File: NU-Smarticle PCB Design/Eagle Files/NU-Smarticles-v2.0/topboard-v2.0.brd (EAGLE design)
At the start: 48 x 22 mm, 17 parts, among them CON1 LI-PO, CON2 12XFFCEXTEND, M1 SERVO, M2 SERVO, U1 XBEE3, U2 INA180B2

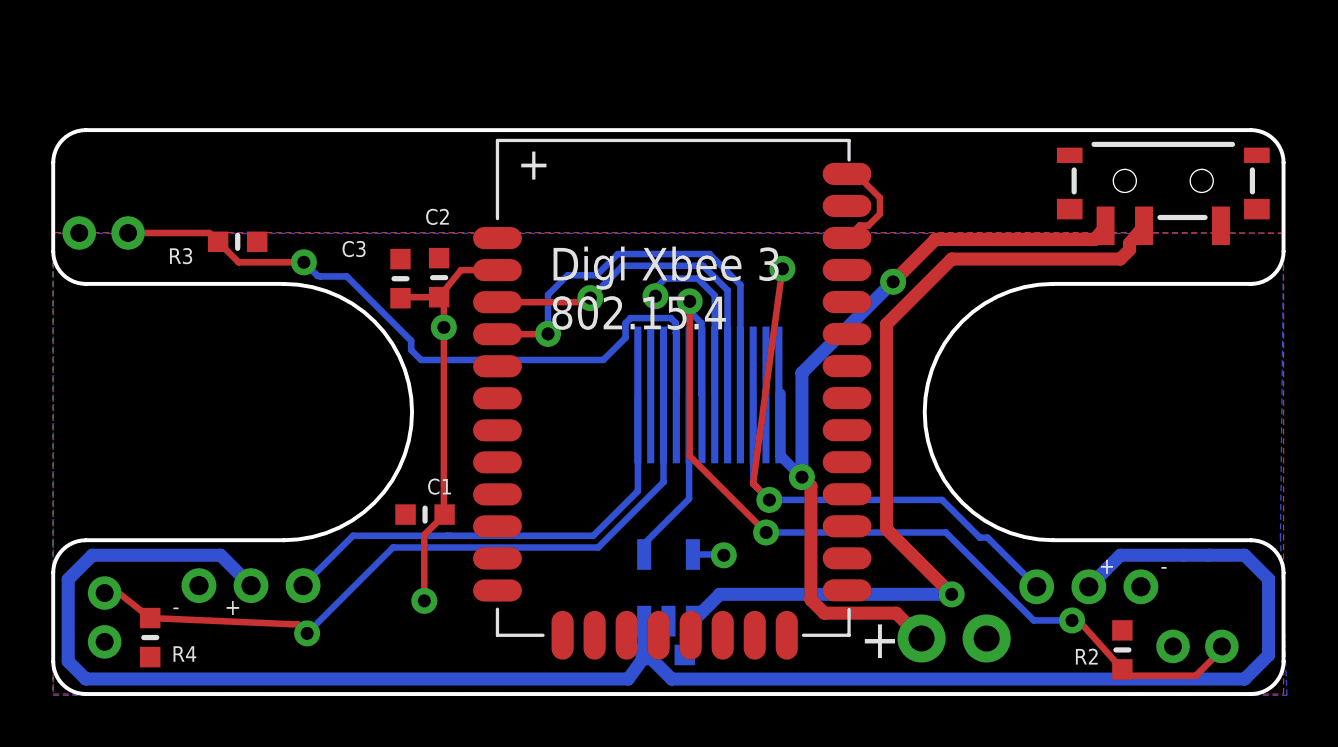
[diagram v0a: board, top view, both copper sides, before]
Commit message: eagle work and files added
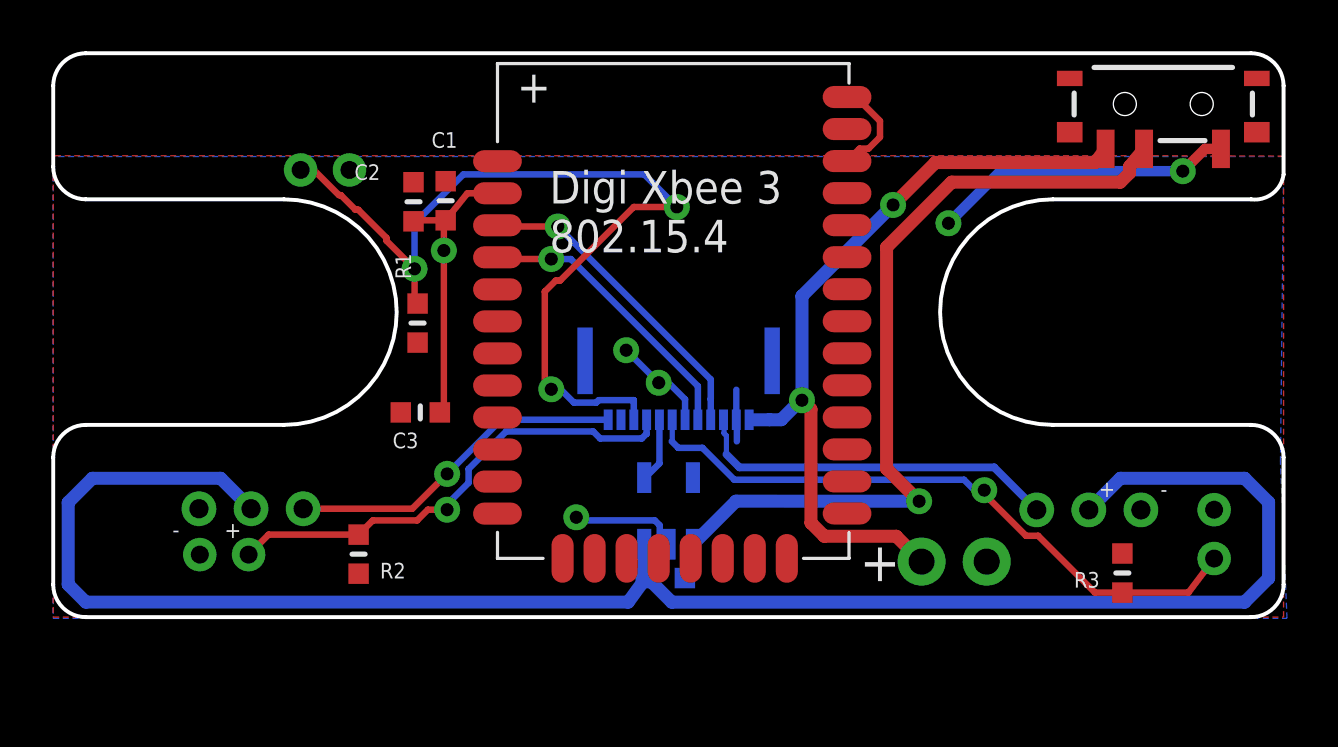
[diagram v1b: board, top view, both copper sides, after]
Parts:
- removed CON2: 12XFFCEXTEND, NU-Smarticle v2:15166-0117_XTEND
- removed R4: 10k, NU-Smarticle v2:_0603MP
- removed U2: INA180B2, NU-Smarticle v2:SOT23-5
- added CON100: 12XFFCMOLEX_51281, NU-Smarticle v2:MOLEX_51281-1294
- added R100: 0.1, NU-Smarticle v2:_0603MP
- added U100: INA180B2, NU-Smarticle v2:SOT23-5
- C1: value 0.1uF -> 9.0pF
- C2: value 9.0pF -> 1.0uF
- C3: value 1.0uF -> 0.1uF
- R1: value 0.1 -> 10k
- moved PH2 45.6 mm to (45.3, 4.19), turned to 270 degrees
- moved PH1 37.1 mm to (11.6, 17.4), turned to 180 degrees
- moved R3 36.9 mm to (41.7, 1.72), turned to 270 degrees
- moved R2 30.0 mm to (11.9, 2.46), turned to 90 degrees
- moved M1 28.8 mm to (9.75, 4.23), turned to 180 degrees
- moved M2 28.8 mm to (38.4, 4.18), turned to 0 degrees
- moved R1 16.2 mm to (14.2, 11.5), flipped to the top, turned to 90 degrees
- moved C1 12.3 mm to (15.3, 16.2), turned to 270 degrees
- moved C3 5.27 mm to (14.3, 7.99), turned to 0 degrees
- moved PH3 5.04 mm to (5.72, 2.44), turned to 0 degrees
- moved C2 3.12 mm to (14.1, 16.2)
- moved CON1 3.00 mm to (33.9, 2.17)
- moved S1 3.00 mm to (43.3, 20.0)
- moved U1 3.00 mm to (24.2, 11.9)
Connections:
- removed net D2: CON2.P7, U1.DOUT/DIO13
- removed net D3: CON2.P8, U1.DIN/CONFIG/DIO14
- removed net D4: CON2.P9, M1.1
- new net D9: CON100.P11, M1.1
- new net RXD1: CON100.P3, U1.DOUT/DIO13
- new net TXD1: CON100.P4, U1.DIN/CONFIG/DIO14
- net 3.3V: now also C1.2, CON100.P1, U100.5; no longer C1.1, CON2.P10, U2.2
- net A0: now also CON100.P6, PH2.2, R3.2; no longer CON2.P5, PH1.2, R2.2
- net A1: now also CON100.P7, U100.4; no longer CON2.P4, U2.4
- net A2: now also CON100.P8, PH3.2, R2.2; no longer CON2.P3, PH2.2, R3.2
- net A3: now also CON100.P9, PH1.2, R1.2; no longer CON2.P2, PH3.2, R4.2
- net D10: now also CON100.P2; no longer CON2.P0
- net GND: now also C1.1, CON100.P5, R1.1, U100.2; no longer C1.2, CON2.P6, R4.1, U2.5
- net N$1: now also R100.2, U100.3; no longer R1.2, U2.3
- net VBAT: now also CON100.P0; no longer CON2.P11
- net VCC_1: now also R100.1, U100.1; no longer R1.1, U2.1
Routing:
- net D4: track 25.5 -> 0.00 mm, vias 2 -> 0
- net D3: track 16.5 -> 0.00 mm, vias 1 -> 0
- net D2: track 14.1 -> 0.00 mm, vias 1 -> 0
- net D9: track 0.00 -> 13.3 mm, vias 0 -> 1
- net RXD1: track 0.00 -> 12.4 mm, vias 0 -> 1
- net GND: track 12.4 -> 24.3 mm, vias 2 -> 5
- net TXD1: track 0.00 -> 11.2 mm, vias 0 -> 1
- net A0: track 34.9 -> 25.2 mm, vias 3 -> 1
- net A2: track 27.5 -> 18.7 mm
- net A3: track 28.1 -> 35.5 mm, vias 1 -> 3
- net A1: track 6.95 -> 2.53 mm
- net D10: track 18.3 -> 14.4 mm
- net 3.3V: track 16.6 -> 13.4 mm, vias 2 -> 1
- net VCC_1: track 35.3 -> 33.2 mm
- net VBAT: track 31.9 -> 30.6 mm
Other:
- outline, holes or cut-outs redrawn
